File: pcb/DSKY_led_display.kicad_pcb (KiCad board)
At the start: 4 copper layers, 63.5 x 107.9 mm, 237 parts, among them J1 105133-0001, J2 20021221-00010C4LF, J3 TSM-104-01-L-SV, Q1 BSS138, Q2 BSS138, Q3 BSS138, Q4 BSS138, SW1 SWITCH_TACT_SMT4.6X2.8, U1 AP2204K-3.3, U2 LP5036, U3 LP5036, U4 LP5036, U5 LP5036, U6 ATSAMD21E18A-A, U7 LP5036, U8 LP5036

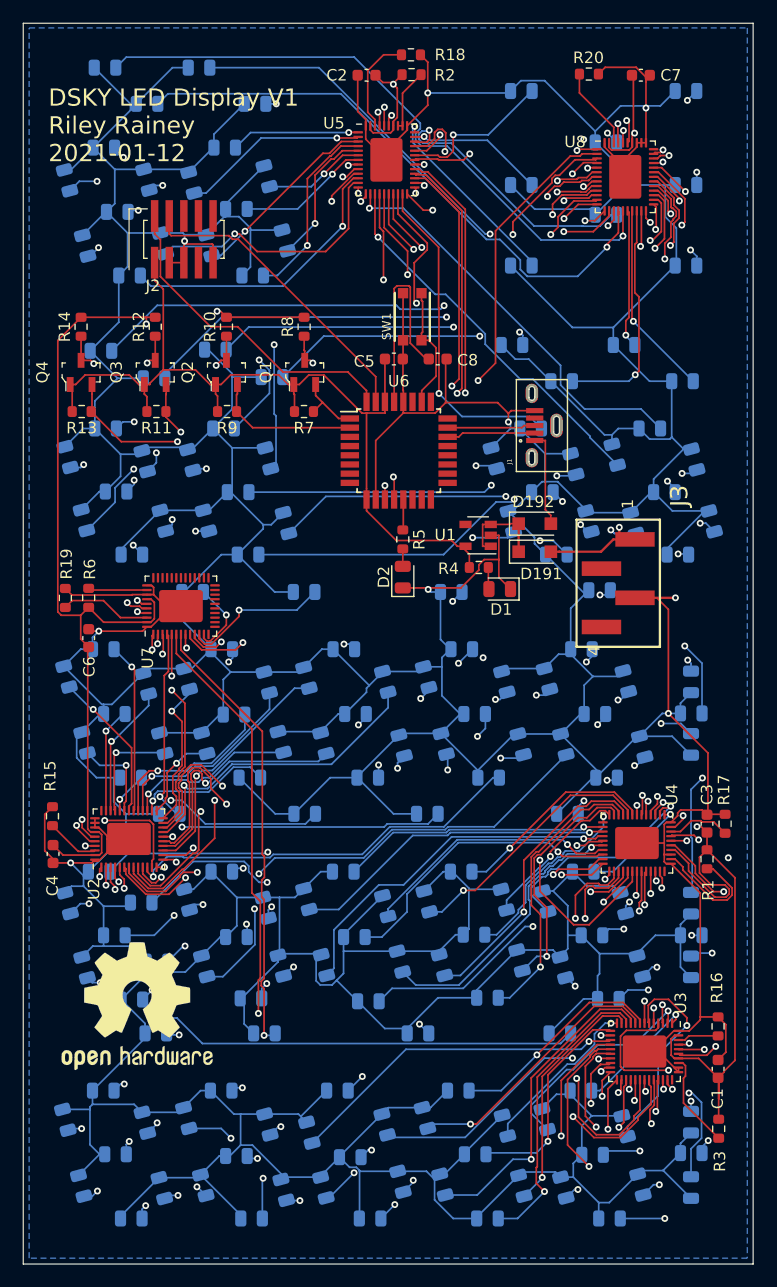
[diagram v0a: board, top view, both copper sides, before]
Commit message: V2 pcb as-ordered for testing
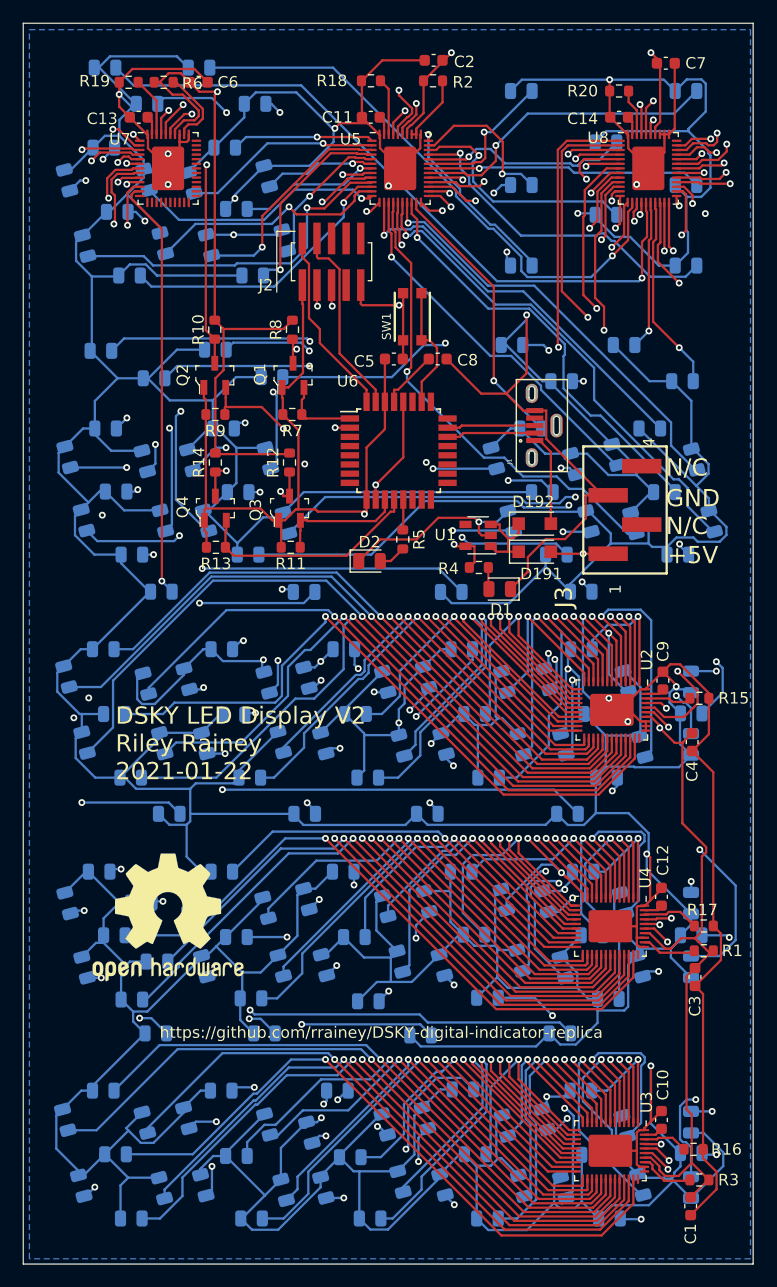
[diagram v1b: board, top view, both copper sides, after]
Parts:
- added C10: 1 uF, Capacitor_SMD:C_0603_1608Metric, F.Cu at (89.4, 128.4)
- added C11: 1 uF, Capacitor_SMD:C_0603_1608Metric, F.Cu at (64.1, 41.1)
- added C12: 1 uF, Capacitor_SMD:C_0603_1608Metric, F.Cu at (89.4, 109.0)
- added C13: 1 uF, Capacitor_SMD:C_0603_1608Metric, F.Cu at (43.9, 41.1)
- added C14: 1 uF, Capacitor_SMD:C_0603_1608Metric, F.Cu at (85.7, 41.1)
- added C9: 1 uF, Capacitor_SMD:C_0603_1608Metric, F.Cu at (89.5, 90.2)
- D191, D192: value D_Schottky -> B0540W
- R15, R16, R17, R18, R19, R20: value 3.7K -> 3.65K
- SW1: value SWITCH_TACT_SMT4.6X2.8 -> KMR241NG
- moved R15 57.2 mm to (92.7, 91.7), turned to 0 degrees
- moved C4 56.4 mm to (92.1, 95.5)
- moved C6 49.3 mm to (49.1, 38.1), turned to 0 degrees
- moved R6 45.3 mm to (46.1, 38.1), turned to 0 degrees
- moved R19 45.2 mm to (43.1, 38.1), turned to 180 degrees
- moved U2 43.5 mm to (85.1, 92.7), turned to 270 degrees
- moved U7 38.1 mm to (46.5, 45.6), turned to 0 degrees
- moved Q4 16.6 mm to (50.6, 75.2)
- moved Q3 16.6 mm to (57.0, 75.2)
- moved R11 16.6 mm to (57.1, 78.6)
- moved R13 16.6 mm to (50.6, 78.6)
- moved R14 16.6 mm to (50.6, 71.2)
- moved R12 16.6 mm to (57.0, 71.2)
- moved C3 13.4 mm to (92.3, 116.0), turned to 270 degrees
- moved J2 13.0 mm to (60.7, 53.7)
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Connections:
- U2 pad 45: +5V -> Net-(C9-Pad1)
- U3 pad 45: +5V -> Net-(C10-Pad1)
- U4 pad 45: +5V -> Net-(C12-Pad1)
- U5 pad 45: +5V -> Net-(C11-Pad1)
- U7 pad 45: +5V -> Net-(C13-Pad1)
- U8 pad 45: +5V -> Net-(C14-Pad1)
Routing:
- net GND: track 1070.7 -> 1396.6 mm, vias 9 -> 34
- net abus30: track 7.82 -> 63.9 mm
- net abus31: track 3.65 -> 58.1 mm
- net g5bus3: track 16.9 -> 69.9 mm, vias 1 -> 2
- net g5bus2: track 29.2 -> 79.5 mm, vias 2 -> 3
- net abus34: track 9.21 -> 59.2 mm
- net abus29: track 13.2 -> 60.2 mm
- net g5bus1: track 41.2 -> 88.0 mm, vias 2 -> 3
- net abus32: track 9.44 -> 55.2 mm
- net g6bus2: track 39.3 -> 84.2 mm, vias 1 -> 2
- net /EN0: track 173.9 -> 129.4 mm, vias 5 -> 6
- net g6bus3: track 36.6 -> 79.6 mm
- net abus33: track 11.6 -> 54.6 mm
- net g6bus1: track 51.6 -> 94.1 mm
- net abus0: track 52.5 -> 11.3 mm, vias 2 -> 1
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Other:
- net class Data: clearance 0.1 -> 0.15; trace_width 0.15 -> 0.2
- net class Default: clearance 0.1 -> 0.15; trace_width 0.15 -> 0.2
- net class GND added: clearance 0.15, trace_width 0.2, via_dia 0.6, via_drill 0.3
- net class Power: clearance 0.1 -> 0.15; trace_width 0.15 -> 0.2
- rule trace_clearance: 0.1 -> 0.15
- board text added: "+5V"
- board text added: "DSKY LED Display V2 Riley Rainey 2021-01-22"
- board text added: "GND"
- board text added: "N/C"
- board text added: "https://github.com/rrainey/DSKY-digital-indicator-replica"
- board text removed: "DSKY LED Display V1 Riley Rainey 2021-01-12"
